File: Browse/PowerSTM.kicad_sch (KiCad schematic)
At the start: 3 parts, among them IC2 TCAN3414DRBR

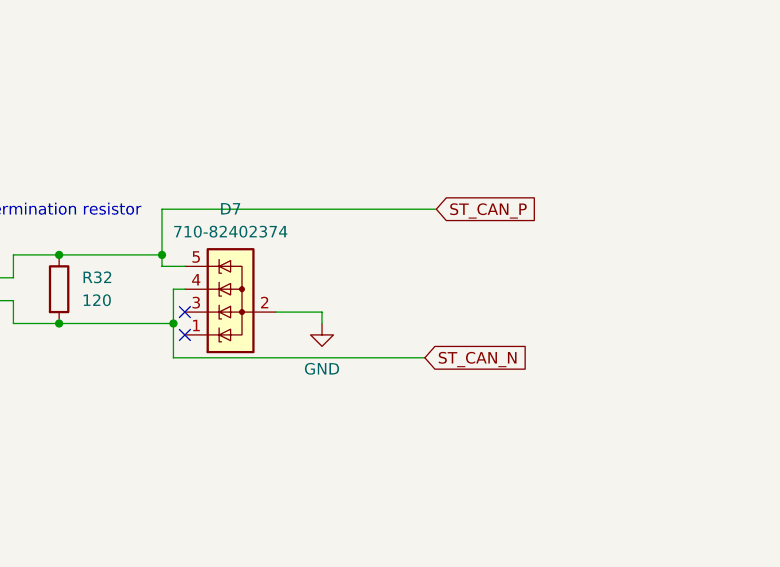
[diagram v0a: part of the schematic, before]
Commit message: Deploying to gh-pages from @ Nautilus-UUV/nautilus-mainboard-PCB@5b07cf6af03655ef9ddad269b1edd5eb03bfa75f 🚀
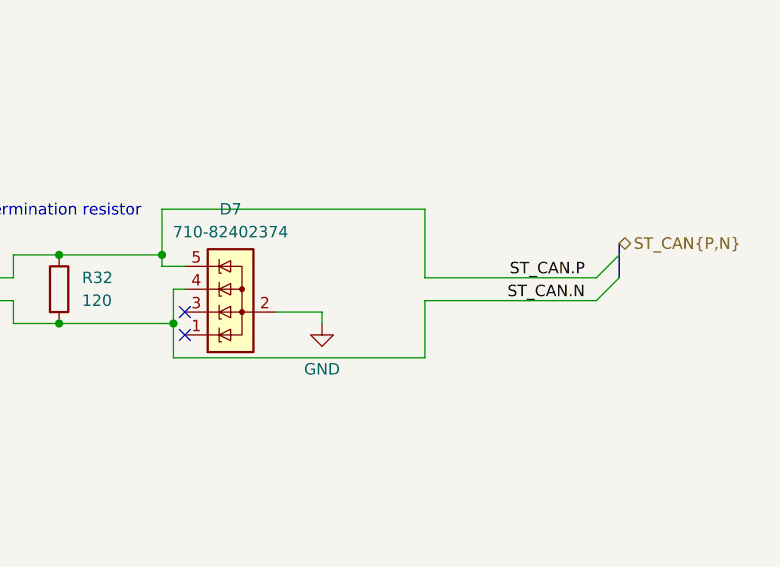
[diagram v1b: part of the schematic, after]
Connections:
- net ST_CAN_N renamed ST_CAN.N
- net ST_CAN_P renamed ST_CAN.P
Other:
- company: Evan -> Evan & Davide
- title: (none) -> Nautilus_Mainboard
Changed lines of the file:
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@@
   (paper "A4")
   (title_block
+    (title "Nautilus_Mainboard")
     (date "2025-11-19")
-    (rev "0")
-    (company "Evan")
+    (rev "1")
+    (company "Evan & Davide")
   )
   (junction (at 196.85 74.93) (diameter 0) (color 0 0 0 0)
@@
   (no_connect (at 199.39 81.28))
   (no_connect (at 199.39 83.82))
+  (bus_entry (at 247.65 74.93) (size -2.54 2.54)
+    (stroke (width 0) (type default))
+  )
+  (bus_entry (at 247.65 77.47) (size -2.54 2.54)
+    (stroke (width 0) (type default))
+  )
+  (wire (pts (xy 226.06 80.01) (xy 245.11 80.01))
+    (stroke (width 0) (type default))
+  )
   (wire (pts (xy 226.06 86.36) (xy 198.12 86.36))
     (stroke (width 0) (type default))
@@
     (stroke (width 0) (type default))
   )
+  (wire (pts (xy 226.06 69.85) (xy 226.06 77.47))
+    (stroke (width 0) (type default))
+  )
   (wire (pts (xy 185.42 82.55) (xy 180.34 82.55))
     (stroke (width 0) (type default))
@@
     (stroke (width 0) (type default))
   )
-  (wire (pts (xy 227.33 69.85) (xy 196.85 69.85))
+  (wire (pts (xy 121.92 80.01) (xy 127 80.01))
     (stroke (width 0) (type default))
   )
-  (wire (pts (xy 121.92 80.01) (xy 127 80.01))
+  (wire (pts (xy 226.06 69.85) (xy 196.85 69.85))
     (stroke (width 0) (type default))
   )
@@
     (stroke (width 0) (type default))
   )
+  (wire (pts (xy 226.06 86.36) (xy 226.06 80.01))
+    (stroke (width 0) (type default))
+  )
   (wire (pts (xy 142.24 102.87) (xy 142.24 99.06))
+    (stroke (width 0) (type default))
+  )
+  (bus (pts (xy 247.65 74.93) (xy 247.65 77.47))
     (stroke (width 0) (type default))
   )
@@
     (stroke (width 0) (type default))
   )
+  (wire (pts (xy 226.06 77.47) (xy 245.11 77.47))
+    (stroke (width 0) (type default))
+  )
   (wire (pts (xy 127 90.17) (xy 127 91.44))
+    (stroke (width 0) (type default))
+  )
+  (bus (pts (xy 247.65 73.66) (xy 247.65 74.93))
     (stroke (width 0) (type default))
   )
@@
     (effects (font (size 1.27 1.27)) (justify right bottom))
   )
-  (global_label "ST_CAN_N" (shape input) (at 226.06 86.36 0) (fields_autoplaced)
+  (label "ST_CAN.N" (at 243.84 80.01 180)
+    (effects (font (size 1.27 1.27)) (justify right bottom))
+  )
+  (label "ST_CAN.P" (at 243.84 77.47 180)
+    (effects (font (size 1.27 1.27)) (justify right bottom))
+  )
+  (hierarchical_label "ST_CAN{P,N}" (shape bidirectional) (at 247.65 73.66 0)
     (effects (font (size 1.27 1.27)) (justify left))
-    (property "Intersheetrefs" "${INTERSHEET_REFS}" (at 238.1771 86.36 0)
-      (effects (font (size 1.27 1.27)) (justify left) (hide yes))
-    )
-  )
-  (global_label "ST_CAN_P" (shape input) (at 227.33 69.85 0) (fields_autoplaced)
-    (effects (font (size 1.27 1.27)) (justify left))
-    (property "Intersheetrefs" "${INTERSHEET_REFS}" (at 239.3866 69.85 0)
-      (effects (font (size 1.27 1.27)) (justify left) (hide yes))
-    )
   )
   (hierarchical_label "FDCAN_STM_RX" (shape output) (at 121.92 80.01 180)

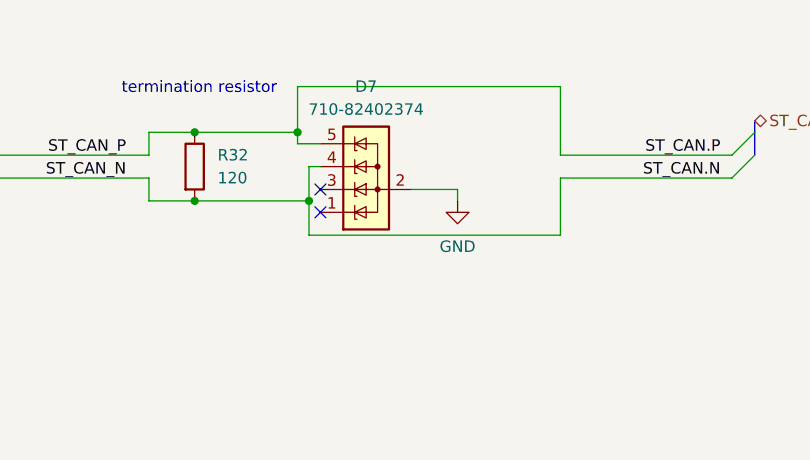
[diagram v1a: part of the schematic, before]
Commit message: Deploying to gh-pages from @ Nautilus-UUV/nautilus-mainboard-PCB@62d9beca31554f779583bfc3c938b3f82a581309 🚀
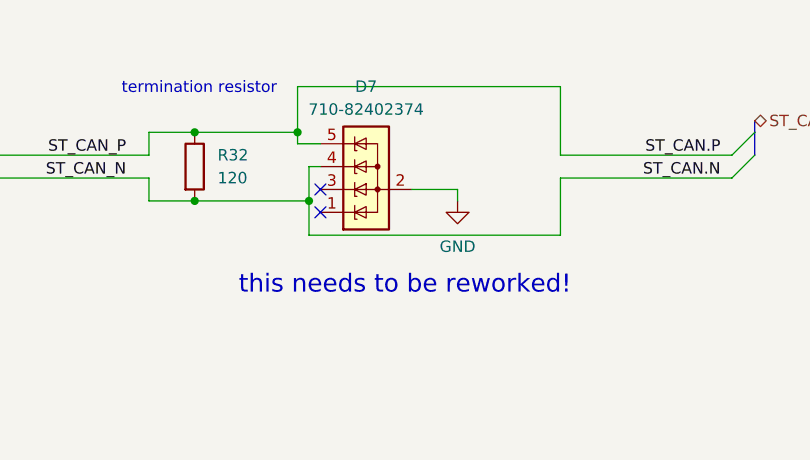
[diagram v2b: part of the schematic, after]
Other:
- note added: "this needs to be reworked!"
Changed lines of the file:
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@@
     (effects (font (size 1.27 1.27)))
+  )
+  (text "this needs to be reworked!" (exclude_from_sim no) (at 208.788 91.948 0)
+    (effects (font (size 2 2) (color 255 36 4 1)))
   )
   (label "ST_CAN_P" (at 177.8 77.47 180)
